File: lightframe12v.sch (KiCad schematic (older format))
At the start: 44 parts, among them J1 PJ-077, J2 Conn_01x06_Female, J3 Conn_01x02_Female, J4 Conn_01x06_Female, J5 Conn_01x04_Female, J6 Conn_01x6_Female, Q1 MMBT2222A-TP, Q2 MMBT2222A-TP, SW1 SW_Push, SW2 SW_Push, U1 TPS562211, U2 ESP32-WROOM-32U, U3 TLC5971

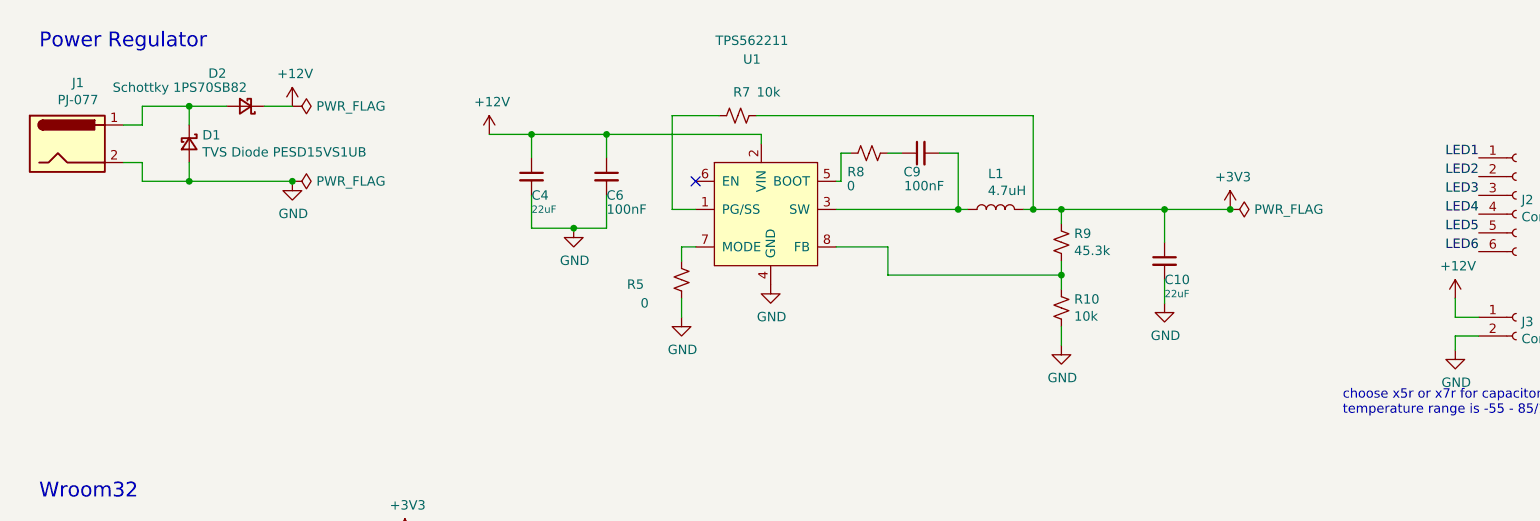
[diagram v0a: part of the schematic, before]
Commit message: Pmic refactor.
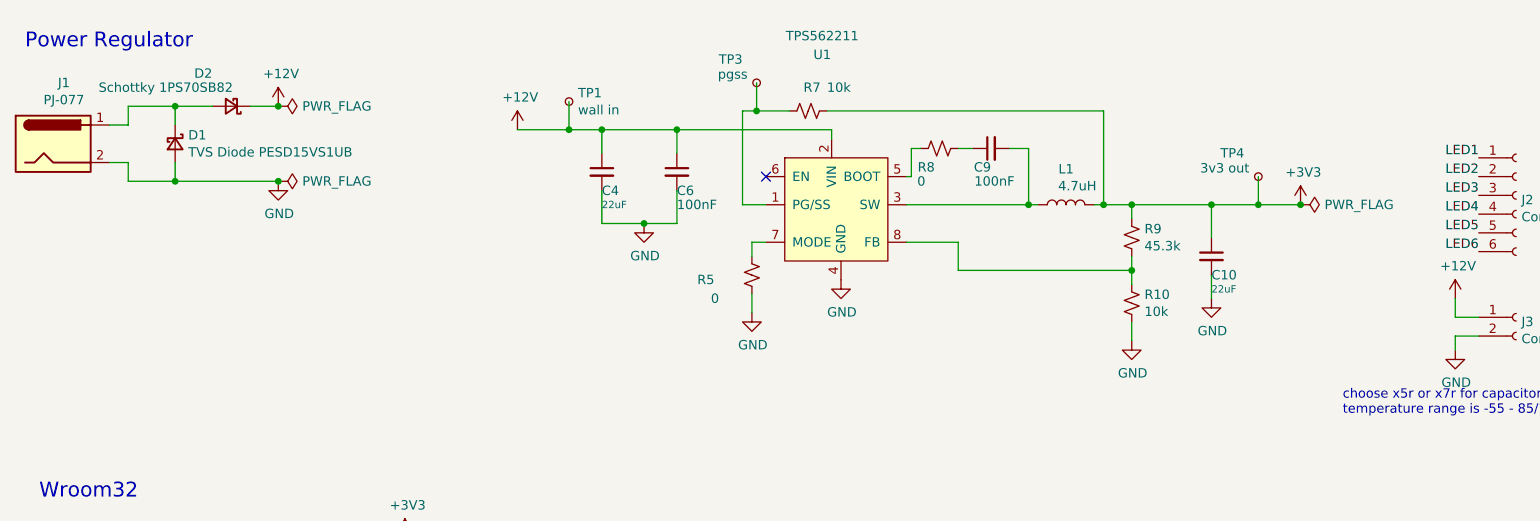
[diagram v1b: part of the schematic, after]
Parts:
- added TP1: wall in, TestPoint:TestPoint_Pad_1.5x1.5mm, symbol Connector:TestPoint_Small
- added TP3: pgss, TestPoint:TestPoint_Pad_1.5x1.5mm, symbol Connector:TestPoint_Small
- added TP4: 3v3 out, TestPoint:TestPoint_Pad_1.5x1.5mm, symbol Connector:TestPoint_Small
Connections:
- net +12V: now also TP1.1
- net +3V3: now also TP4.1
- net at R7.2, U1.1 (PG/SS): now also TP3.1
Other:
- moved on the sheet: C10, C4, C6, C9, D1, D2, J1, L1, R10, R5, R7, R8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
